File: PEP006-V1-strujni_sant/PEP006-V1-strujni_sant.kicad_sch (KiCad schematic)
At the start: 15 parts, among them J1 Screw_Terminal_01x02

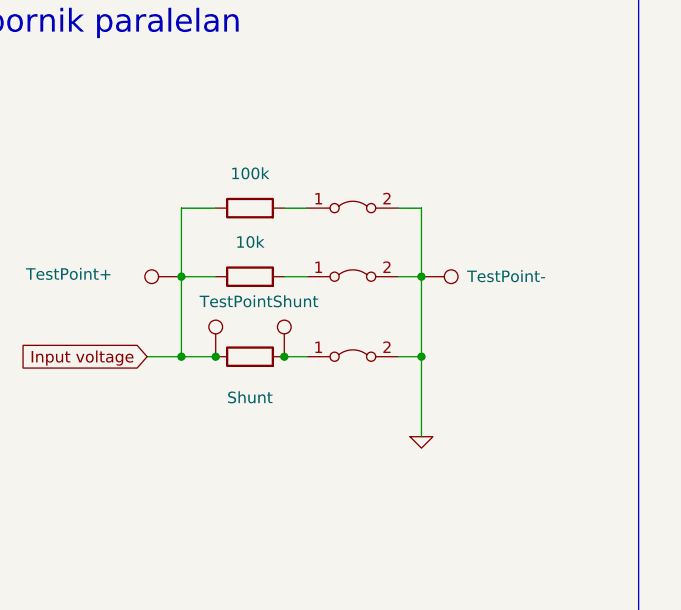
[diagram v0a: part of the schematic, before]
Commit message: PEP006 update.
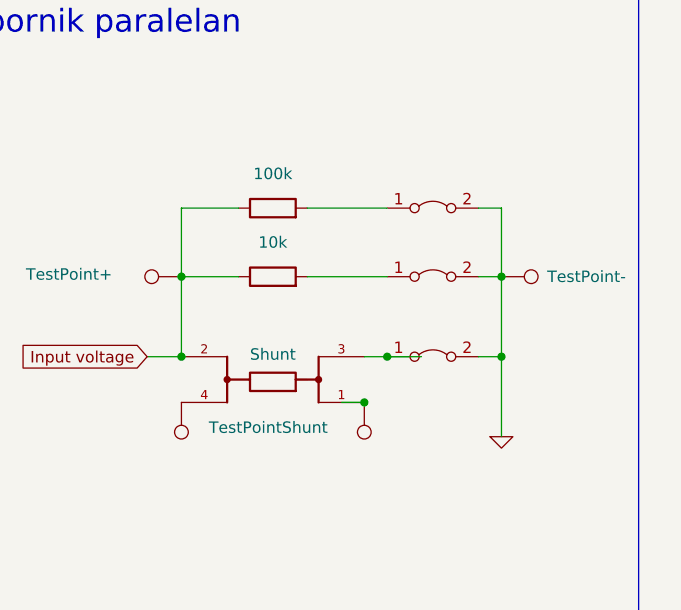
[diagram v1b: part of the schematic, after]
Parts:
- removed R5: Shunt, WSK12161L000FEA (1):RES_WSK12161L000FEA, symbol Device:R
- added R1: Shunt, WSK12161L000FEA (1):RES_WSK12161L000FEA, symbol WSK12161L000FEA:WSK12161L000FEA
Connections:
- net Input voltage: now also R1.2; no longer TP6.1
- net at TP7.1: now also R1.1; no longer JP3.1 (A)
- new net: JP3.1 (A), R1.3
- new net: R1.4, TP6.1
